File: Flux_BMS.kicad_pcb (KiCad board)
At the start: 4 copper layers, 90 x 65 mm, 221 parts, among them J1 Conn_01x02, J2 Conn_01x02, J3 USB_C_Receptacle_USB2.0, J4 CAN, J5 Conn_01x16, J7 Conn_01x05, J8 Conn_01x05, Q14 YJG30N06A, Q15 Q_NMOS_SDG, Q18 BST82,215, U1 BQ76940DBT, U2 STM32L476RGTx, U3 BQ76200PW, U4 INA180A2, U5 TJA1051T-3, U6 USBLC6-2SC6, U8 ME6118A33, U9 LM5164DDA, X1 8MHz(16pF)

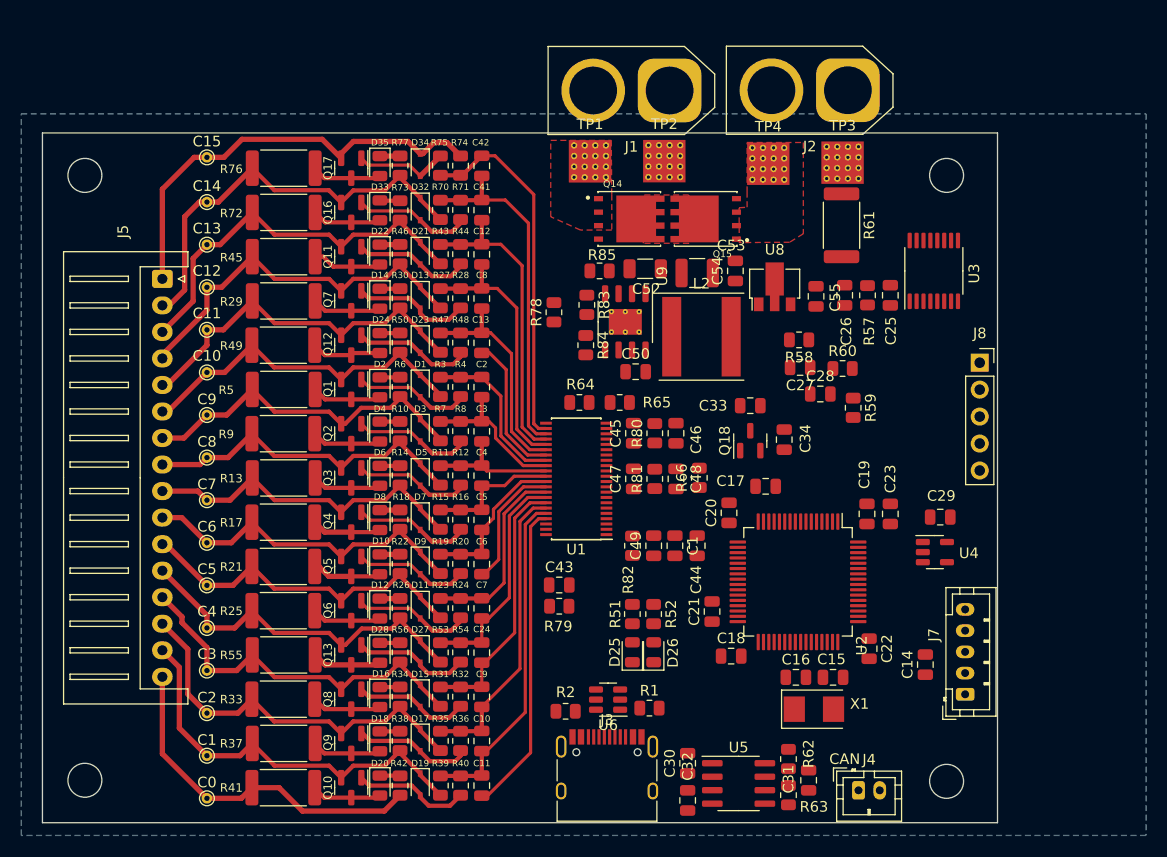
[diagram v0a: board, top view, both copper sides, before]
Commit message: almost ready to order
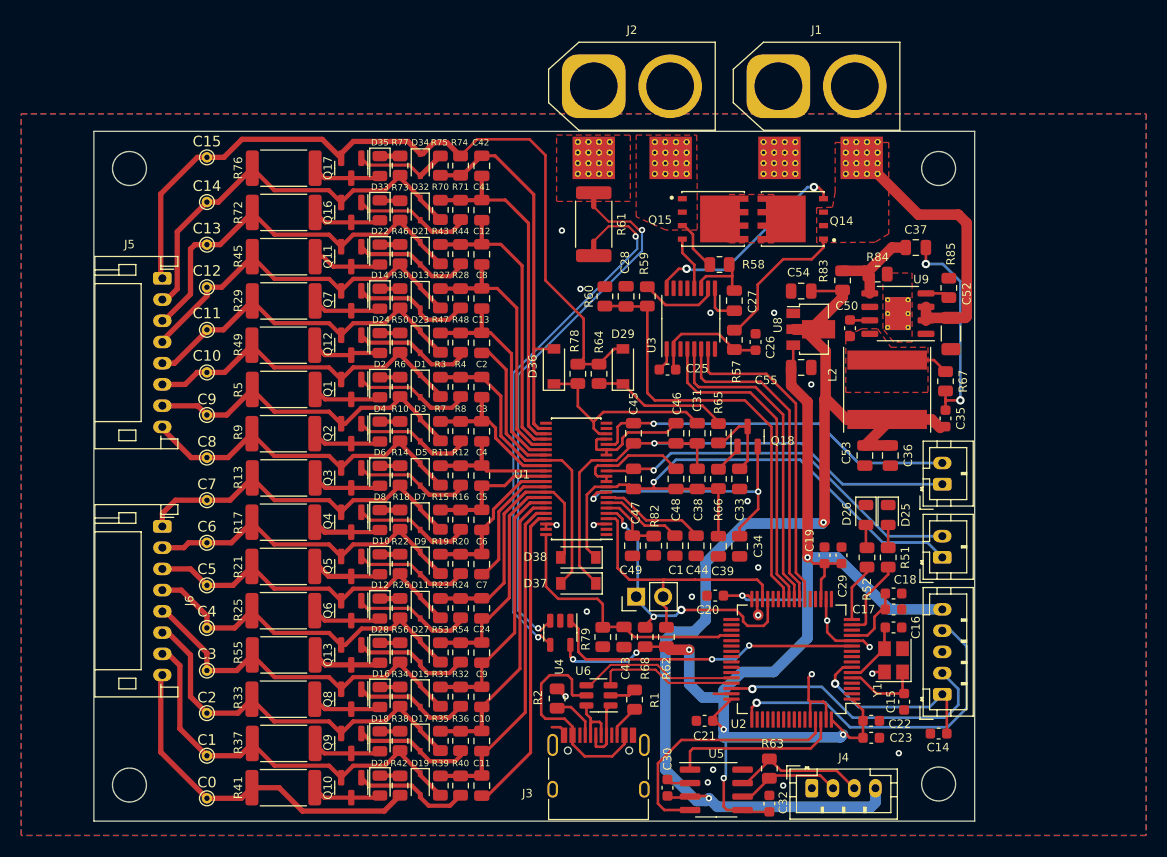
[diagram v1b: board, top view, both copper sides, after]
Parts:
- removed X1: 8MHz(16pF), Crystal:Crystal_SMD_5032-2Pin_5.0x3.2mm
- added C35: 1n2, Capacitor_SMD:C_0603_1608Metric, F.Cu at (156.2, 100.6)
- added C36: 22u, Capacitor_SMD:C_0805_2012Metric, F.Cu at (151.1, 104.1)
- added C37: 47p, Capacitor_SMD:C_0805_2012Metric, F.Cu at (153.4, 84.5)
- added C38: 10u, Capacitor_SMD:C_0805_2012Metric, F.Cu at (132.8, 106.3)
- added C39: 10u, Capacitor_SMD:C_0805_2012Metric, F.Cu at (134.8, 112.7)
- added D29: 100V, Diode_SMD:D_SOD-123, F.Cu at (125.8, 95.7)
- added D36: 100V, Diode_SMD:D_SOD-123, F.Cu at (119.3, 95.7)
- added D37: 100V, Diode_SMD:D_SOD-123, F.Cu at (121.7, 116.2)
- added D38: 100V, Diode_SMD:D_SOD-123, F.Cu at (121.7, 113.7)
- added J6: Conn_01x08, Connector_JST:JST_PH_S8B-PH-K_1x08_P2.00mm_Horizontal, F.Cu at (82.5, 110.8)
- added NT1: NetTie_2, NetTie:NetTie-2_SMD_Pad0.5mm, F.Cu at (123.1, 80.2)
- added NT2: NetTie_2, NetTie:NetTie-2_SMD_Pad0.5mm, F.Cu at (123.1, 84.4)
- added R67: 237k, Resistor_SMD:R_0805_2012Metric, F.Cu at (156.2, 97.1)
- added R68: 10k, Resistor_SMD:R_0805_2012Metric, F.Cu at (128.0, 121.2)
- added Y1: 8Mhz, Crystal:Crystal_SMD_3225-4Pin_3.2x2.5mm, F.Cu at (151.3, 123.4)
- C10, C11, C12, C13, C2, C24, C3, C4, C41, C42, C5, C6, C7, C8, C9: value ~ -> 220n
- C14: value C -> 100n; footprint Capacitor_SMD:C_0805_2012Metric -> Capacitor_SMD:C_0603_1608Metric
- C15, C16: value 20p -> 15p; footprint Capacitor_SMD:C_0805_2012Metric -> Capacitor_SMD:C_0603_1608Metric
- C17, C18, C19, C20, C21, C22, C26, C29, C30, C32, C50: footprint Capacitor_SMD:C_0805_2012Metric -> Capacitor_SMD:C_0603_1608Metric
- C23: value 4,7u -> 4u7; footprint Capacitor_SMD:C_0805_2012Metric -> Capacitor_SMD:C_0603_1608Metric
- C25: value 470n -> 1u; footprint Capacitor_SMD:C_0805_2012Metric -> Capacitor_SMD:C_0603_1608Metric
- C31: value 1n -> 10u
- C53: footprint Capacitor_SMD:C_1210_3225Metric -> Capacitor_SMD:C_0805_2012Metric
- J4: footprint Connector_JST:JST_PH_B2B-PH-K_1x02_P2.00mm_Vertical -> Connector_JST:JST_PH_B4B-PH-K_1x04_P2.00mm_Vertical
- J5: value Conn_01x16 -> Conn_01x08; footprint Connector_JST:JST_XH_S16B-XH-A_1x16_P2.50mm_Horizontal -> Connector_JST:JST_PH_S8B-PH-K_1x08_P2.00mm_Horizontal
- J8: value Conn_01x05 -> Conn_01x02; footprint Connector_PinSocket_2.54mm:PinSocket_1x05_P2.54mm_Vertical -> Connector_PinHeader_2.54mm:PinHeader_1x02_P2.54mm_Vertical
- L2: value 33u -> 68u
- Q14: value YJG30N06A -> HYG025N06LS1C2
- Q15: value Q_NMOS_SDG -> HYG025N06LS1C2
- R51, R52: value 100 -> 220
- R62: value 56 -> 10k
- R63: value 56 -> 120
- R80, R81: footprint Resistor_SMD:R_0805_2012Metric -> Connector_JST:JST_PH_B2B-PH-K_1x02_P2.00mm_Vertical
- R83: value 316k -> 453k
- R84: value 101k -> 49k9
- R85: value 41k2 -> 100k
- moved J8 39.2 mm to (127.1, 117.4), turned to 90 degrees
- moved U4 36.1 mm to (120.0, 120.8), turned to -90 degrees
- moved C31 34.3 mm to (132.8, 102.0)
- moved R85 33.0 mm to (156.6, 88.3), turned to 90 degrees
- moved C52 29.5 mm to (156.8, 92.6), turned to -90 degrees
- moved R84 28.3 mm to (149.8, 87.0), turned to 0 degrees
- moved R81 28.1 mm to (155.9, 113.7)
- moved R80 27.5 mm to (155.9, 106.8)
- moved D25 27.4 mm to (150.8, 109.7), turned to -90 degrees
- moved TP1 26.2 mm to (148.3, 79.0), turned to 180 degrees
- moved U9 25.7 mm to (151.8, 90.7), turned to 180 degrees
- moved R51 24.7 mm to (150.8, 113.7), turned to 90 degrees
- moved R83 24.2 mm to (146.6, 87.6), turned to 90 degrees
- moved TP3 24.1 mm to (123.1, 79.0), turned to 180 degrees
- moved J2 24.0 mm to (123.1, 69.3), turned to 0 degrees
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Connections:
- net /BQ76940/Cell1/SENSE- renamed /BQ76940/VC0
- net /BQ76940/SENSE+_1 renamed /BQ76940/VC1
- net /BQ76940/SENSE+_10 renamed /BQ76940/VC10
- net /BQ76940/SENSE+_11 renamed /BQ76940/VC11
- net /BQ76940/SENSE+_12 renamed /BQ76940/VC12
- net /BQ76940/SENSE+_13 renamed /BQ76940/VC13
- net /BQ76940/SENSE+_14 renamed /BQ76940/VC14
- net /BQ76940/SENSE+_15 renamed /BQ76940/VC15
- net /BQ76940/SENSE+_2 renamed /BQ76940/VC2
- net /BQ76940/SENSE+_3 renamed /BQ76940/VC3
- net /BQ76940/SENSE+_4 renamed /BQ76940/VC4
- net /BQ76940/SENSE+_5 renamed /BQ76940/VC5
- net /BQ76940/SENSE+_6 renamed /BQ76940/VC6
- net /BQ76940/SENSE+_7 renamed /BQ76940/VC7
- net /BQ76940/SENSE+_8 renamed /BQ76940/VC8
- net /BQ76940/SENSE+_9 renamed /BQ76940/VC9
- net /STM32L476/USB_DM renamed /STM32L476/USB_DN
- C31 pad 1: Net-(C31-Pad1) -> /BQ76940/VC15X
- C31 pad 2: GND -> /BQ76940/VC10X
- J3 pad A4: unconnected-(J3-PadA4) -> Net-(J3-PadA4)
- J3 pad A9: unconnected-(J3-PadA4) -> Net-(J3-PadA4)
- J3 pad B4: unconnected-(J3-PadA4) -> Net-(J3-PadA4)
- J3 pad B9: unconnected-(J3-PadA4) -> Net-(J3-PadA4)
- J4 pad 1: /CAN/CAN_H -> GND
- J7 pad 1: +3V3 -> /STM32L476/NRST
- J7 pad 2: /STM32L476/NRST -> /STM32L476/SWDIO
- J7 pad 3: /STM32L476/SWCLK -> GND
- J7 pad 4: /STM32L476/SWDIO -> /STM32L476/SWCLK
- J7 pad 5: GND -> +3V3
- J8 pad 1: /Charge_control/BQ_CHG_EN -> /BQ76940/BQ_SCL
- J8 pad 2: /Charge_control/BQ_CP_EN -> /BQ76940/BQ_SDA
- R61 pad 1: Net-(R61-Pad1) -> Net-(NT1-Pad1)
- R62 pad 1: /CAN/CAN_H -> +3V3
- R62 pad 2: Net-(C31-Pad1) -> /BQ76940/BQ_SDA
- R63 pad 1: Net-(C31-Pad1) -> /CAN/CAN_H
- R78 pad 1: /BQ76940/BAT -> /BQ76940/VC15X
- TP3 pad 1: Net-(R61-Pad1) -> Net-(NT1-Pad1)
- U1 pad 20: /BQ76940/BAT -> /BQ76940/VC15X
- U2 pad 11: unconnected-(U2-Pad11) -> /Charge_control/CHARGER_CUR
- U2 pad 15: unconnected-(U2-Pad15) -> /STM32L476/LED_RED
- U2 pad 16: unconnected-(U2-Pad16) -> /STM32L476/LED_GREEN
- U2 pad 20: /STM32L476/LTC_CS -> unconnected-(U2-Pad20)
- U2 pad 21: /STM32L476/LTC_SCK -> unconnected-(U2-Pad21)
- U2 pad 22: /STM32L476/LTC_SDO -> /Charge_control/BQ_PMON_EN
- U2 pad 23: /STM32L476/LTC_SDI -> /Charge_control/BQ_DSG_EN
- U2 pad 24: unconnected-(U2-Pad24) -> /Charge_control/BQ_CP_EN
- U2 pad 25: unconnected-(U2-Pad25) -> /Charge_control/BQ_CHG_EN
- U2 pad 26: unconnected-(U2-Pad26) -> /Charge_control/CHARGER_V
- U2 pad 29: unconnected-(U2-Pad29) -> /BQ76940/BQ_SCL
- U2 pad 30: /Charge_control/BQ_PMON_EN -> /BQ76940/BQ_SDA
- U2 pad 33: /Charge_control/BQ_PCHG_EN -> unconnected-(U2-Pad33)
- U2 pad 34: /Charge_control/BQ_CP_EN -> unconnected-(U2-Pad34)
- U2 pad 35: /Charge_control/BQ_DSG_EN -> unconnected-(U2-Pad35)
- U2 pad 36: /Charge_control/BQ_CHG_EN -> /BQ76940/BQ_ALERT
- U2 pad 42: /STM32L476/LED_RED -> unconnected-(U2-Pad42)
- U2 pad 43: /STM32L476/LED_GREEN -> unconnected-(U2-Pad43)
- U2 pad 46: /STM32L476/SWCLK -> /STM32L476/SWDIO
- U2 pad 49: /STM32L476/SWDIO -> /STM32L476/SWCLK
- U2 pad 58: /STM32L476/CURRENT_MEASURE_EN -> unconnected-(U2-Pad58)
- U2 pad 60: unconnected-(U2-Pad60) -> GND
- U3 pad 8: /Charge_control/BQ_PCHG_EN -> unconnected-(U3-Pad8)
- U4 pad 1: unconnected-(U4-Pad1) -> /Charge_control/CHARGER_CUR
- U4 pad 3: Net-(R61-Pad1) -> /Charge_control/CUR_+
- U4 pad 4: GND -> /Charge_control/CUR_-
- U6 pad 2: unconnected-(U6-Pad2) -> GND
- U6 pad 5: unconnected-(U6-Pad5) -> Net-(J3-PadA4)
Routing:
- net +3V3: track 0.00 -> 128.5 mm, vias 0 -> 8
- net +5V: track 0.00 -> 109.9 mm, vias 0 -> 2
- net /BQ76940/VC5X: track 0.00 -> 56.2 mm, vias 0 -> 1
- net /BQ76940/VC10X: track 0.00 -> 54.4 mm, vias 0 -> 1
- net /Charge_control/CUR_+: track 0.00 -> 50.3 mm, vias 0 -> 2
- net /Charge_control/CUR_-: track 0.00 -> 50.3 mm, vias 0 -> 2
- net /Charge_control/CHARGER_V: track 0.00 -> 41.9 mm
- net V+: track 0.00 -> 39.1 mm
- net /BQ76940/TS2: track 0.00 -> 35.7 mm, vias 0 -> 1
- net /BQ76940/C15: track 41.6 -> 77.0 mm
- net /BQ76940/TS3: track 0.00 -> 34.9 mm, vias 0 -> 1
- net GND: track 0.00 -> 33.8 mm, vias 0 -> 21
- net /STM32L476/SWCLK: track 0.00 -> 32.0 mm, vias 0 -> 1
- net /Charge_control/BQ_CP_EN: track 0.00 -> 30.6 mm
- net /Charge_control/BQ_CHG_EN: track 0.00 -> 30.5 mm
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- added copper zone on F.Cu, net /Power/SW
- added copper zone on F.Cu, net GND
- added copper zone on F.Cu, net Net-(NT1-Pad1)
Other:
- board size 90 x 65 mm -> 83 x 65 mm
